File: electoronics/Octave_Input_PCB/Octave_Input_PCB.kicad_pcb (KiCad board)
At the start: 2 copper layers, 95.2 x 95.2 mm, 28 parts, among them SW1 SW_Hot_Swap_Socket, SW10 SW_Hot_Swap_Socket, SW11 SW_Hot_Swap_Socket, SW12 SW_Hot_Swap_Socket, SW13 SW_Hot_Swap_Socket, SW14 SW_Hot_Swap_Socket, SW2 SW_Hot_Swap_Socket, SW3 SW_Hot_Swap_Socket, SW4 SW_Hot_Swap_Socket, SW5 SW_Hot_Swap_Socket, SW6 SW_Hot_Swap_Socket, SW7 SW_Hot_Swap_Socket, SW8 SW_Hot_Swap_Socket, SW9 SW_Hot_Swap_Socket

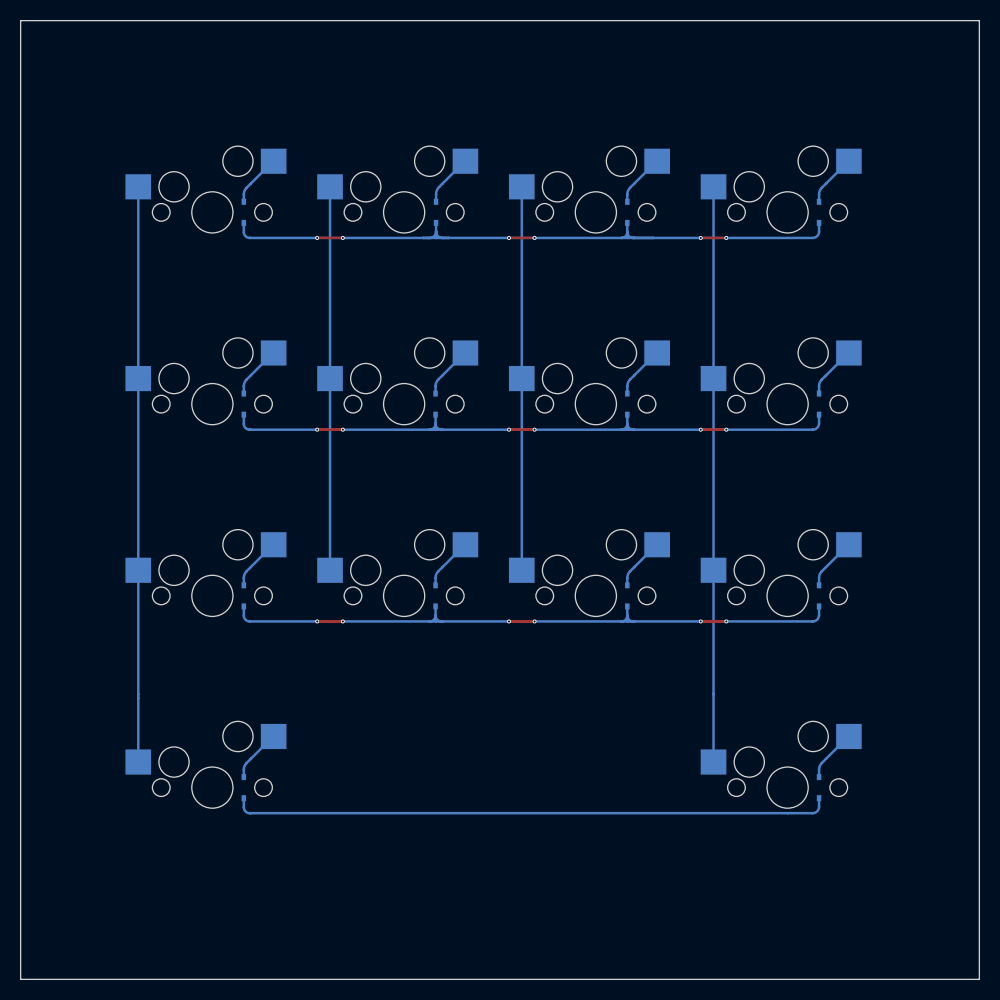
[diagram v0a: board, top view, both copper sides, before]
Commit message: Update schematic
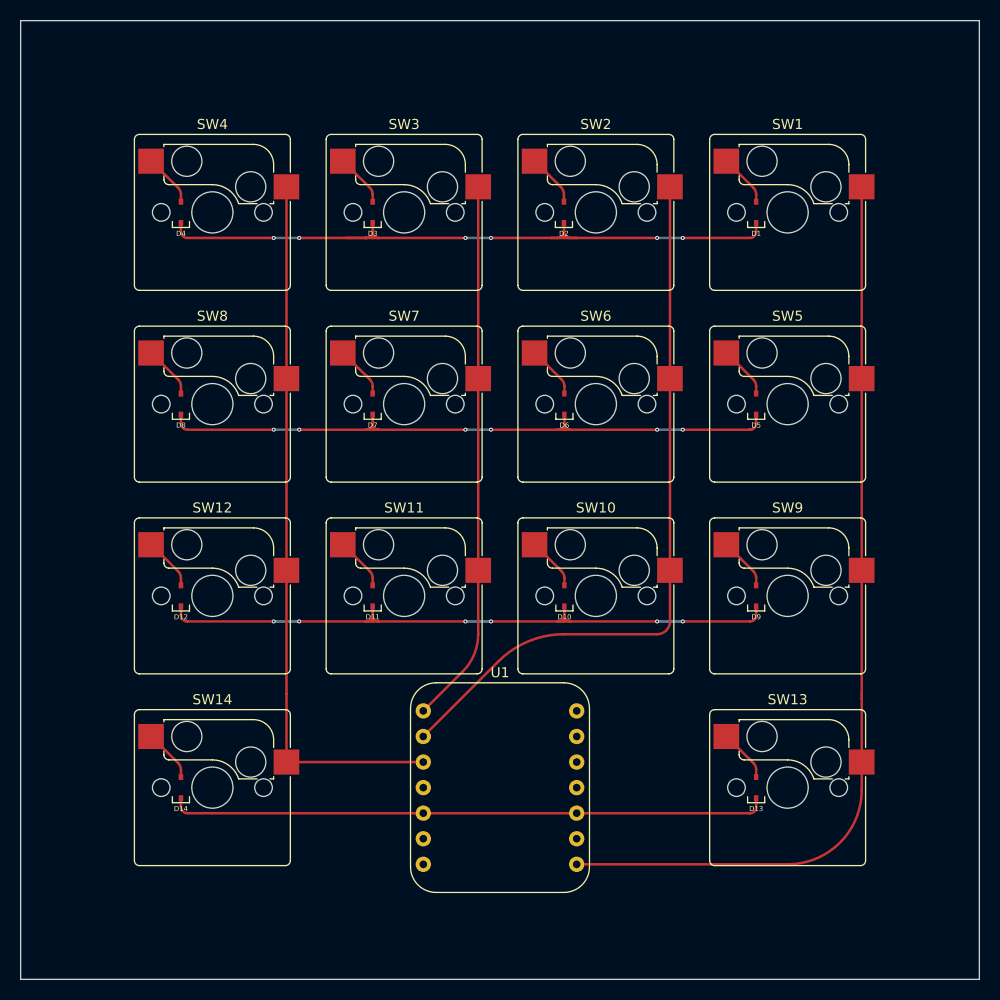
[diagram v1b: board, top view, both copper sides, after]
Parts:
- added U1: Adafruit_QT_Py_RP2040, Octave_Library:Adafruit_QT_Py_RP2040, F.Cu at (85.7, 114.3)
- D1, D10, D11, D12, D13, D14, D2, D3, D4, D5, D6, D7, D8, D9, SW1, SW10, SW11, SW12, SW13, SW14, SW2, SW3, SW4, SW5, SW6, SW7, SW8, SW9: moved to F.Cu
- moved D12 63.4 mm to (54.0, 95.2)
- moved D14 63.4 mm to (54.0, 114.3)
- moved D4 63.4 mm to (54.0, 57.1)
- moved D8 63.4 mm to (54.0, 76.2)
- moved SW1 57.1 mm to (114.3, 57.1), turned to 0 degrees
- moved SW12 57.1 mm to (57.1, 95.2), turned to 0 degrees
- moved SW13 57.1 mm to (114.3, 114.3), turned to 0 degrees
- moved SW14 57.1 mm to (57.1, 114.3), turned to 0 degrees
- moved SW4 57.1 mm to (57.1, 57.1), turned to 0 degrees
- moved SW5 57.1 mm to (114.3, 76.2), turned to 0 degrees
- moved SW8 57.1 mm to (57.1, 76.2), turned to 0 degrees
- moved SW9 57.1 mm to (114.3, 95.2), turned to 0 degrees
- moved D1 50.9 mm to (111.2, 57.1)
- moved D13 50.9 mm to (111.2, 114.3)
- moved D5 50.9 mm to (111.2, 76.2)
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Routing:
- net col0: track 57.2 -> 92.2 mm
- net col1: track 38.1 -> 72.1 mm
- net col2: track 38.1 -> 54.1 mm
- net col3: track 57.2 -> 70.7 mm
